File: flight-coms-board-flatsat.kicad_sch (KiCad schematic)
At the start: 57 parts, among them J1 DIN41612_02x05_ZB_EvenPins, J2 SMA-10V21-TGG, U1 CC1200, U2 TPS79330-EP, Y2 40MHz, Y3 TG-5021CG

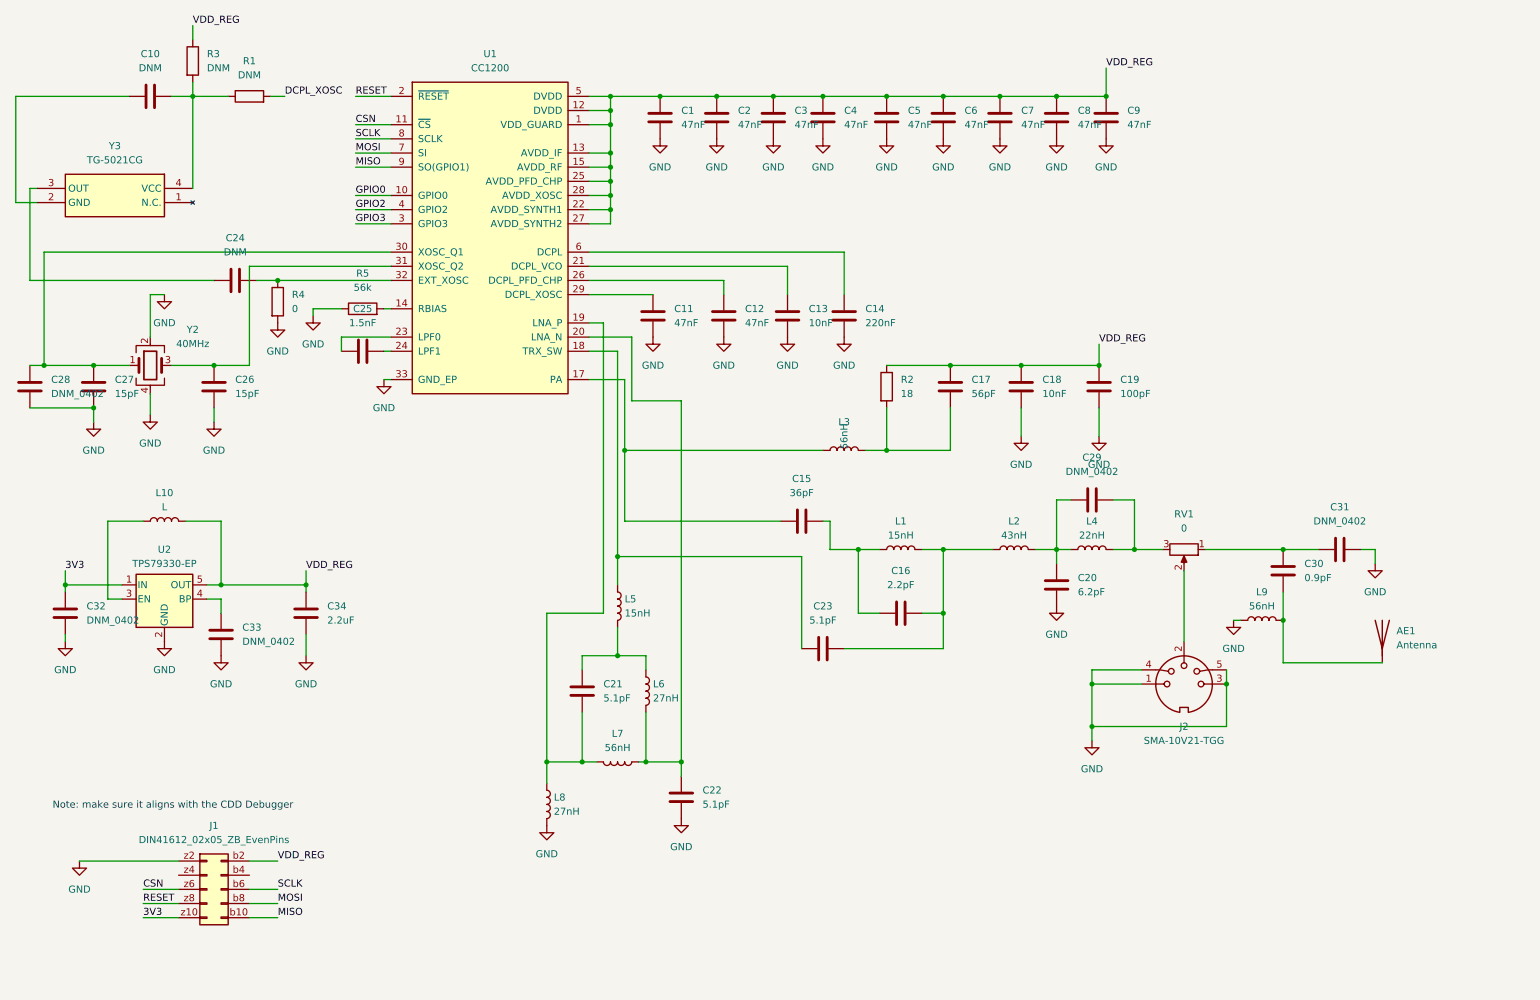
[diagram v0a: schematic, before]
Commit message: Add files via upload
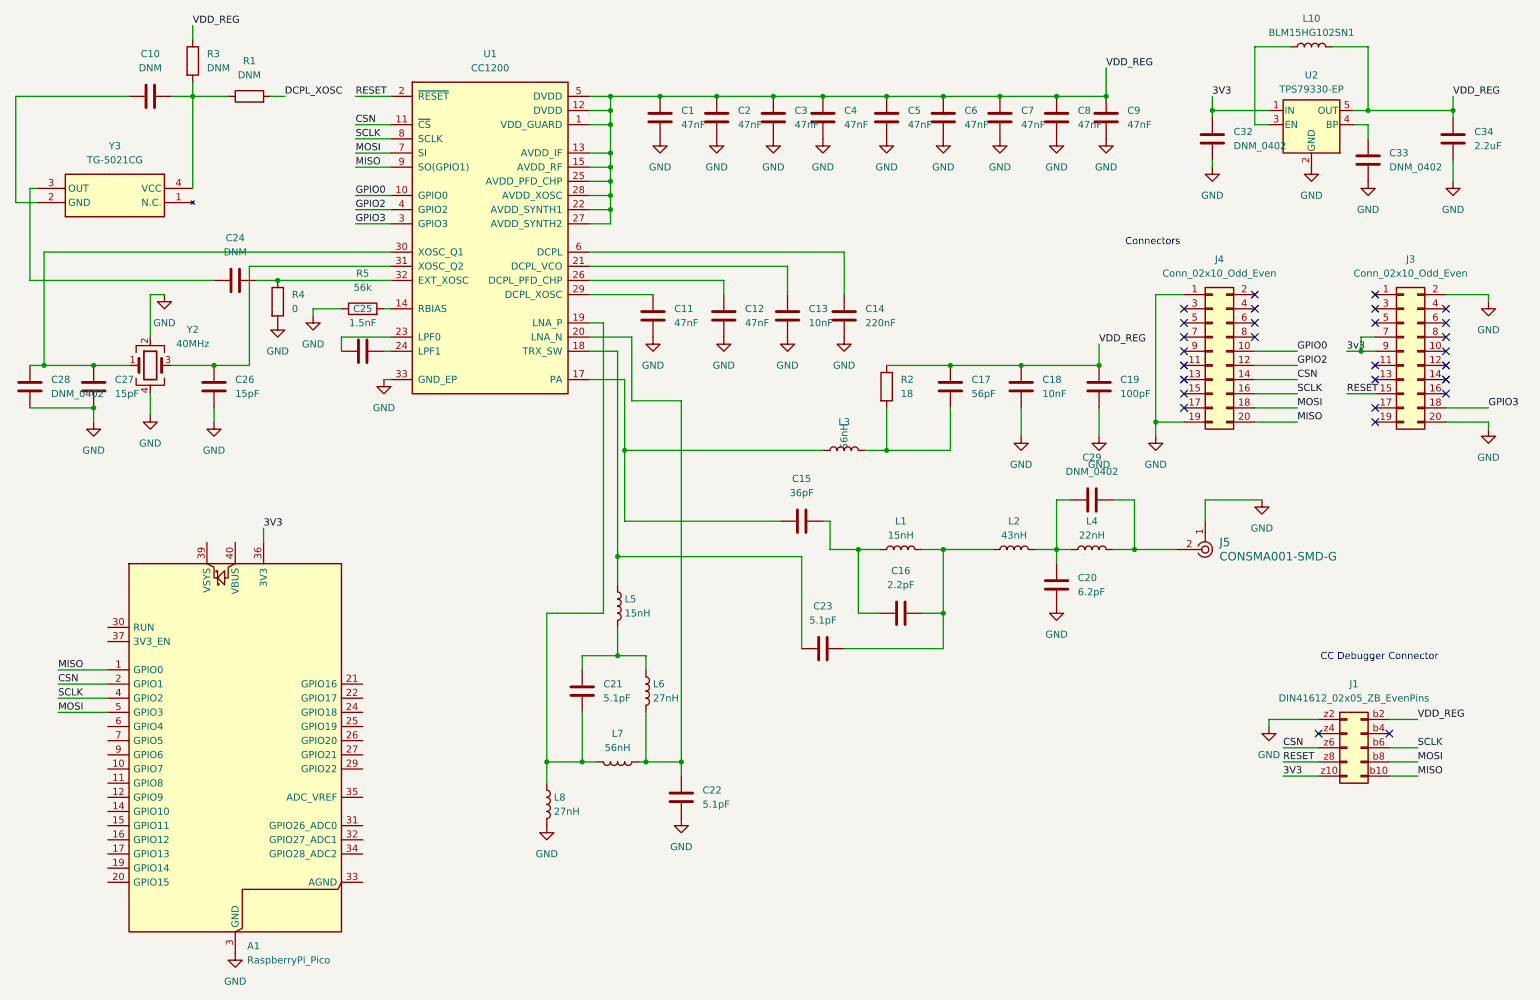
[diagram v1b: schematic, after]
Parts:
- removed AE1: Antenna, symbol Device:Antenna
- removed C30: 0.9pF, symbol Device:C
- removed C31: DNM_0402, symbol Device:C
- removed J2: SMA-10V21-TGG, symbol Connector:DIN-5_180degree
- removed L9: 56nH, symbol Device:L
- removed RV1: 0, symbol Device:R_Potentiometer
- added A1: RaspberryPi_Pico, Module:RaspberryPi_Pico_Common_Unspecified, symbol MCU_Module:RaspberryPi_Pico
- added J3, J4: Conn_02x10_Odd_Even, Connector_PinHeader_1.00mm:PinHeader_2x10_P1.00mm_Vertical_SMD, symbol Connector_Generic:Conn_02x10_Odd_Even
- added J5: CONSMA001-SMD-G, digikey-footprints:RF_SMA_Receptical_Vertical_CONSMA001-SMD-G, symbol dk_Coaxial-Connectors-RF:CONSMA001-SMD-G
- C1, C10, C11, C12, C13, C14, C15, C16, C17, C18, C19, C2, C20, C21, C22, C23, C24, C25, C26, C27, C28, C29, C3, C32, C33, C4, C5, C6, C7, C8, C9, R1, R3: footprint (none) -> Capacitor_SMD:C_0402_1005Metric_Pad0.74x0.62mm_HandSolder
- C34: footprint (none) -> Capacitor_SMD:C_0603_1608Metric_Pad1.08x0.95mm_HandSolder
- J1: footprint (none) -> Connector_PinHeader_1.00mm:PinHeader_2x05_P1.00mm_Vertical_SMD
- L1, L2, L3, L4, L5, L6, L7, L8: footprint (none) -> Inductor_SMD:L_0402_1005Metric_Pad0.77x0.64mm_HandSolder
- L10: value L -> BLM15HG102SN1; footprint (none) -> Inductor_SMD:L_0402_1005Metric_Pad0.77x0.64mm_HandSolder
- R2, R4, R5: footprint (none) -> Resistor_SMD:R_0402_1005Metric_Pad0.72x0.64mm_HandSolder
- Y2: footprint (none) -> Oscillator:Oscillator_SMD_SeikoEpson_SG8002CE-4Pin_3.2x2.5mm
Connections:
- net 3V3: now also A1.36 (3V3)
- net CSN: now also A1.2 (GPIO1), J4.14 (Pin_14)
- net GND: now also A1.13 (GND), A1.18 (GND), A1.23 (GND), A1.28 (GND), A1.3 (GND), A1.38 (GND), A1.8 (GND), J3.2 (Pin_2), J3.20 (Pin_20), J4.1 (Pin_1), J4.19 (Pin_19), J5.1
- net GPIO0: now also J4.10 (Pin_10)
- net GPIO2: now also J4.12 (Pin_12)
- net GPIO3: now also J3.18 (Pin_18)
- net MISO: now also A1.1 (GPIO0), J4.20 (Pin_20)
- net MOSI: now also A1.5 (GPIO3), J4.18 (Pin_18)
- net RESET: now also J3.15 (Pin_15)
- net SCLK: now also A1.4 (GPIO2), J4.16 (Pin_16)
- net at C29.2, L4.2: now also J5.2
- new net 3v3: J3.7 (Pin_7), J3.9 (Pin_9)
- no-connect marks 0 -> 28
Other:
- note added: "CC Debugger Connector"
- note added: "Connectors"
- note removed: "Note: make sure it aligns with the CDD Debugger"
- moved on the sheet: C32, C33, C34, J1, L10, U2
